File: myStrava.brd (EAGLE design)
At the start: 64.8 x 45.4 mm, 43 parts, among them Y1 16MHz

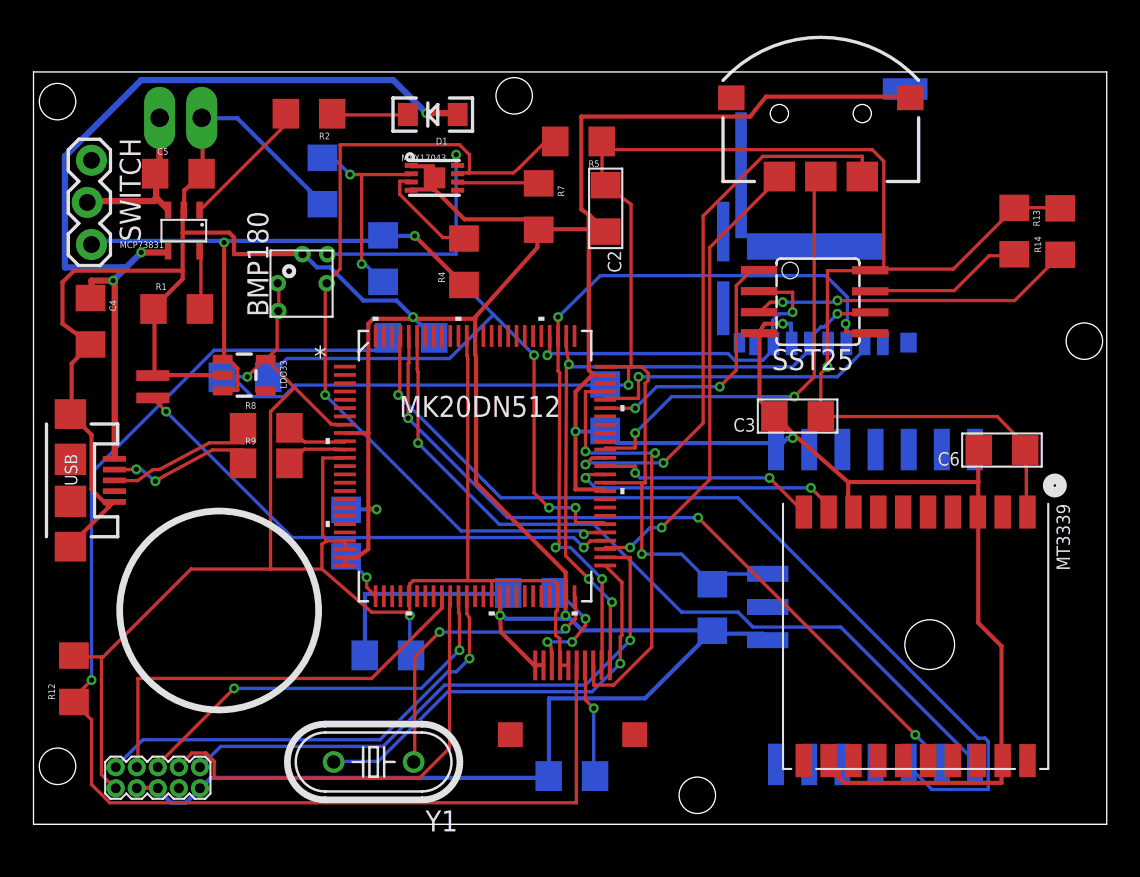
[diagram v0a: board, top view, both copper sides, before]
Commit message: Candidat V2
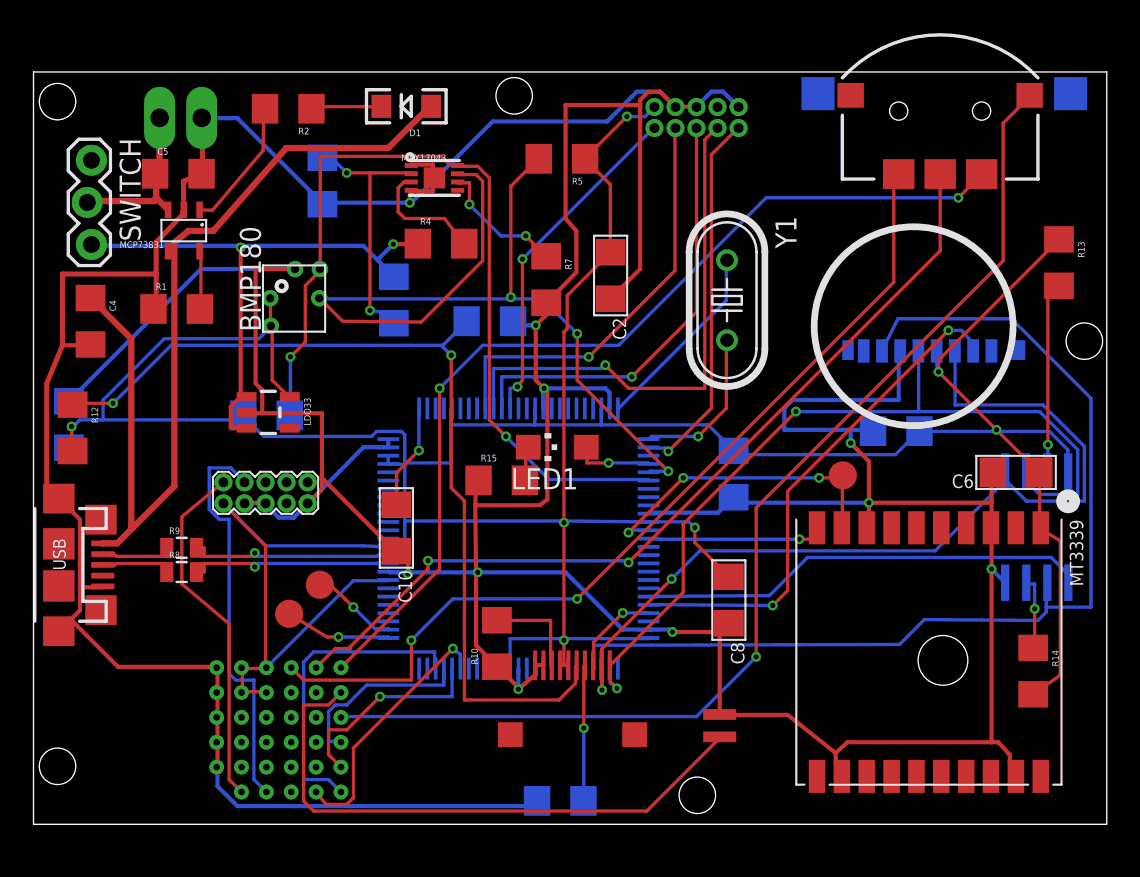
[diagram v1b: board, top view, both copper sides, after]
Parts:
- removed N550: ANTAP28, ANTAP28:ANTAP
- added JTAG1: 2X5_0.05"_CORTEX_DEBUGTH_NOKEY_UNSHROUDED, con-cortex:2X5_0.05"_TH_NS
- added LED1: (no value), adafruit:CHIPLED_1206
- added R15: 180, SparkFun-Resistors:1206
- added U$1: N548, N548:N548
- added U$17: GPS_TX, Exposed_pad:IND-2020
- added U$26: PTE0, Exposed_pad:IND-2020
- added U$32: PTE1, Exposed_pad:IND-2020
- R8, R9: device SparkFun-Resistors:1206 -> SparkFun-Resistors:0805
- moved JTAG 51.4 mm to (40.0, 42.6), flipped to the bottom, turned to 180 degrees
- moved SPK 37.1 mm to (40.4, 6.95), turned to 270 degrees
- moved Y1 35.1 mm to (41.8, 31.6), turned to 270 degrees
- moved R14 26.6 mm to (60.3, 9.24), turned to 270 degrees
- moved C7 23.8 mm to (2.14, 24.1), turned to 90 degrees
- moved SST25 22.4 mm to (58.0, 13.1), flipped to the bottom, turned to 90 degrees
- moved R12 15.1 mm to (2.36, 23.9), turned to 270 degrees
- moved R8 10.1 mm to (8.94, 15.2)
- moved C9 8.72 mm to (42.2, 21.1)
- moved R9 7.21 mm to (8.94, 16.7)
- moved NAV 7.20 mm to (54.7, 43.0)
- moved SD 6.57 mm to (55.0, 35.2)
- moved C3 6.02 mm to (52.0, 23.7), flipped to the bottom, turned to 0 degrees
- moved USB 5.15 mm to (1.53, 15.7)
- moved MK20DN512 5.10 mm to (29.3, 17.2), flipped to the bottom, turned to 180 degrees
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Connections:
- removed net MK_RX3: MK20DN512.95, N550.TX
- removed net MK_TX3: MK20DN512.96, N550.RX
- removed net VDD: BMP180.VDD, BMP180.VDDIO, C2.1, C3.1, C6.1, C7.1, C8.1, C9.1, JTAG.1, LDO33.5, MK20DN512.12, MK20DN512.22, MK20DN512.23, MK20DN512.30, MK20DN512.40, MK20DN512.48, MK20DN512.61, MK20DN512.75, MK20DN512.8, MK20DN512.89, MT3339.P$1, N550.VCC, R12.2, R13.1, R14.2, R5.1, R6.1, SD.VCC, SHARP.VDD, SHARP.VDDA, SST25.VDD
- new net N$10: SPK.P$2, U$1.P002
- new net N$11: MK20DN512.96, U$1.P005
- new net N$12: MK20DN512.95, U$1.P009
- new net N$13: MK20DN512.97, U$1.P003
- new net N$15: MK20DN512.98, U$1.P008
- new net N$24: MK20DN512.2, U$32.P$1
- new net N$28: JTAG1.2, U$1.SWDIO
- new net N$5: NAV.T, U$1.P030
- new net N$6: NAV.1, U$1.P024
- new net N$9: NAV.C, U$1.P001
- new net VCC: BMP180.VDD, BMP180.VDDIO, C2.1, C3.1, C6.1, C7.1, C8.1, C9.1, JTAG.1, JTAG1.1, LDO33.5, MK20DN512.12, MK20DN512.22, MK20DN512.23, MK20DN512.30, MK20DN512.40, MK20DN512.48, MK20DN512.61, MK20DN512.75, MK20DN512.8, MK20DN512.89, MT3339.P$1, R12.2, R13.1, R14.2, R5.1, R6.1, SD.VCC, SHARP.VDD, SHARP.VDDA, SST25.VDD, U$1.B5, U$1.B6, U$1.C5, U$1.C6
- net GND: now also JTAG1.3, JTAG1.5, JTAG1.9, R15.1, SPK.P$1, U$1.A2, U$1.A3, U$1.A4, U$1.A5, U$1.A6; no longer N550.GND, N550.GND2, NAV.C, SPK.P$2
- net MK_RX1: now also U$17.P$1
- net N$21: now also MK20DN512.1, U$26.P$1; no longer MK20DN512.97, N550.BR1
- net N$29: now also JTAG1.4, U$1.SWDCLK; no longer MK20DN512.64, NAV.2
- net N$3: now also NAV.2, U$1.P031; no longer MK20DN512.54, SPK.P$1
- net N$30: now also LED1.A, MK20DN512.54; no longer MK20DN512.65, NAV.T
- net N$31: now also LED1.C, R15.2; no longer MK20DN512.53, NAV.1
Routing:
- net VCC: track 0.00 -> 244.0 mm, vias 0 -> 7
- net VDD: track 236.5 -> 0.00 mm, vias 5 -> 0
- net N$9: track 0.00 -> 67.3 mm, vias 0 -> 1
- net N$6: track 0.00 -> 54.7 mm, vias 0 -> 2
- net N$5: track 0.00 -> 53.1 mm, vias 0 -> 2
- net N$21: track 56.3 -> 6.43 mm
- net MK_RX3: track 48.2 -> 0.00 mm, vias 1 -> 0
- net MK_TX3: track 45.9 -> 0.00 mm, vias 3 -> 0
- net MK_DI: track 21.8 -> 62.5 mm, vias 2 -> 0
- net N$10: track 0.00 -> 35.6 mm
- net GND: track 341.7 -> 371.8 mm, vias 7 -> 10
- net N$3: track 31.2 -> 57.4 mm
- net N$31: track 28.1 -> 2.08 mm, vias 2 -> 0
- net N$27: track 78.9 -> 56.0 mm, vias 1 -> 2
- net N$30: track 27.2 -> 4.73 mm, vias 2 -> 1
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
